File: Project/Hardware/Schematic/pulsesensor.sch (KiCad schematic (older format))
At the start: 2 parts, among them U4 Pulse_sensor

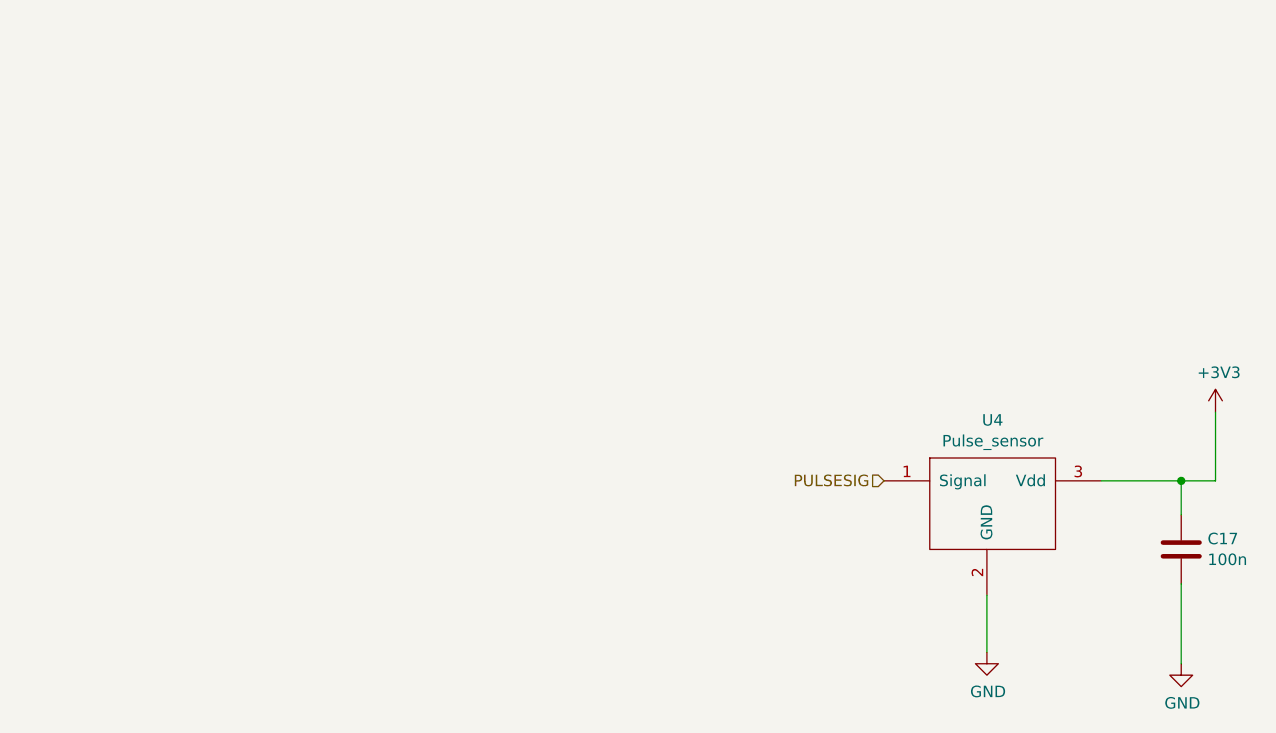
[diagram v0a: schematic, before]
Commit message: Intermediate...
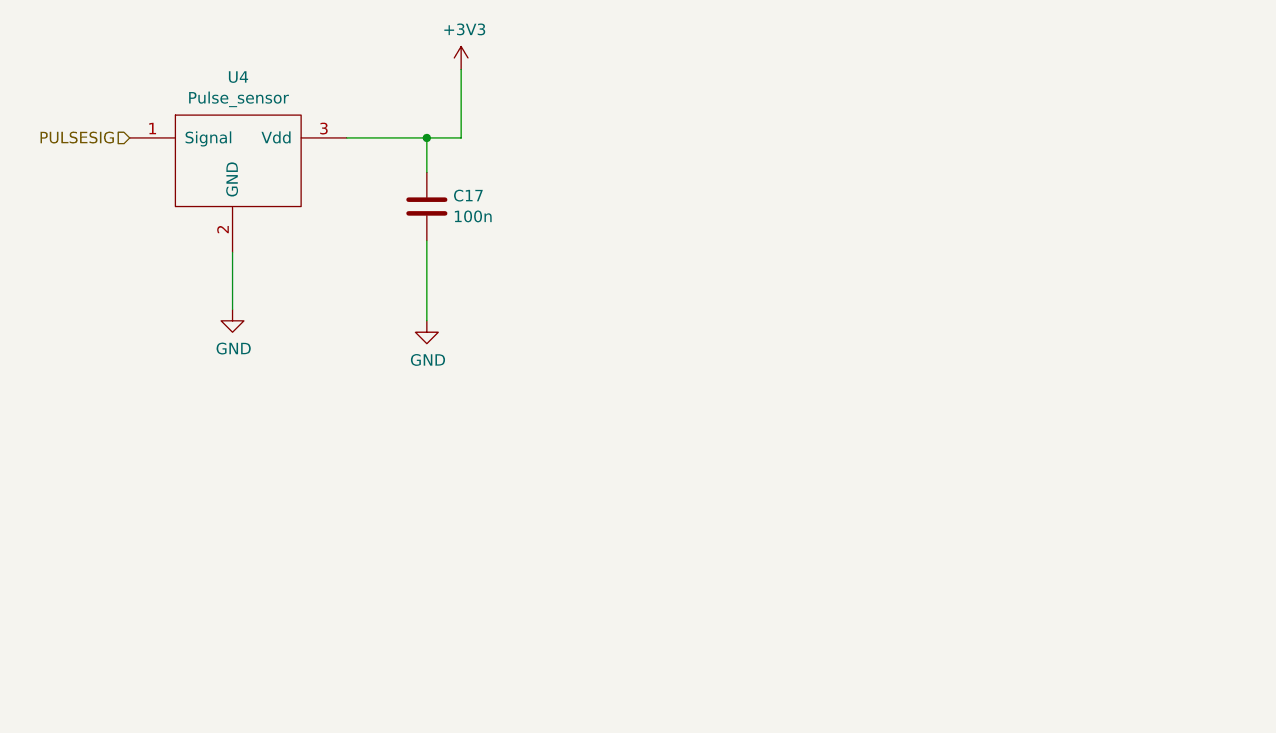
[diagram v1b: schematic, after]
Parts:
- C17: footprint (none) -> Capacitor_SMD:C_0805_2012Metric_Pad1.15x1.40mm_HandSolder
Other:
- moved on the sheet: C17, U4
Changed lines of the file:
@@
 EELAYER 26 0
 EELAYER END
-$Descr A4 11693 8268
+$Descr User 5512 5512
 encoding utf-8
 Sheet 3 7
 Title ""
-Date ""
-Rev ""
-Comp ""
+Date "2019-02-12"
+Rev "1"
+Comp "PASC"
 Comment1 ""
 Comment2 ""
@@
 L PASC:Pulse_sensor U4
 U 1 1 5C5DA663
-P 5700 3400
-F 0 "U4" H 5725 3765 50  0000 C CNN
-F 1 "Pulse_sensor" H 5725 3674 50  0000 C CNN
-F 2 "Pin_Headers:Pin_Header_Straight_1x03_Pitch2.54mm" H 5700 3400 50  0001 C CNN
-F 3 "" H 5700 3400 50  0001 C CNN
-	1    5700 3400
+P 2400 1900
+F 0 "U4" H 2425 2265 50  0000 C CNN
+F 1 "Pulse_sensor" H 2425 2174 50  0000 C CNN
+F 2 "Pin_Headers:Pin_Header_Straight_1x03_Pitch2.54mm" H 2400 1900 50  0001 C CNN
+F 3 "" H 2400 1900 50  0001 C CNN
+	1    2400 1900
 	1    0    0    -1
 $EndComp
@@
 L power:+3V3 #PWR0125
 U 1 1 5C5DA797
-P 6700 3000
-F 0 "#PWR0125" H 6700 2850 50  0001 C CNN
-F 1 "+3V3" H 6715 3173 50  0000 C CNN
-F 2 "" H 6700 3000 50  0001 C CNN
-F 3 "" H 6700 3000 50  0001 C CNN
-	1    6700 3000
+P 3400 1500
+F 0 "#PWR0125" H 3400 1350 50  0001 C CNN
+F 1 "+3V3" H 3415 1673 50  0000 C CNN
+F 2 "" H 3400 1500 50  0001 C CNN
+F 3 "" H 3400 1500 50  0001 C CNN
+	1    3400 1500
 	1    0    0    -1
 $EndComp
@@
 L Device:C C17
 U 1 1 5C5DA7DA
-P 6550 3600
-F 0 "C17" H 6665 3646 50  0000 L CNN
-F 1 "100n" H 6665 3555 50  0000 L CNN
-F 2 "" H 6588 3450 50  0001 C CNN
-F 3 "~" H 6550 3600 50  0001 C CNN
-	1    6550 3600
+P 3250 2100
+F 0 "C17" H 3365 2146 50  0000 L CNN
+F 1 "100n" H 3365 2055 50  0000 L CNN
+F 2 "Capacitor_SMD:C_0805_2012Metric_Pad1.15x1.40mm_HandSolder" H 3288 1950 50  0001 C CNN
+F 3 "~" H 3250 2100 50  0001 C CNN
+	1    3250 2100
 	1    0    0    -1
 $EndComp
 Wire Wire Line
-	6200 3300 6550 3300
+	2900 1800 3250 1800
 Wire Wire Line
-	6700 3300 6700 3000
+	3400 1800 3400 1500
 $Comp
 L power:GND #PWR0126
 U 1 1 5C5DA906
-P 5700 4050
-F 0 "#PWR0126" H 5700 3800 50  0001 C CNN
-F 1 "GND" H 5705 3877 50  0000 C CNN
-F 2 "" H 5700 4050 50  0001 C CNN
-F 3 "" H 5700 4050 50  0001 C CNN
-	1    5700 4050
+P 2400 2550
+F 0 "#PWR0126" H 2400 2300 50  0001 C CNN
+F 1 "GND" H 2405 2377 50  0000 C CNN
+F 2 "" H 2400 2550 50  0001 C CNN
+F 3 "" H 2400 2550 50  0001 C CNN
+	1    2400 2550
 	1    0    0    -1
 $EndComp
@@
 L power:GND #PWR0127
 U 1 1 5C5DA96D
-P 6550 4100
-F 0 "#PWR0127" H 6550 3850 50  0001 C CNN
-F 1 "GND" H 6555 3927 50  0000 C CNN
-F 2 "" H 6550 4100 50  0001 C CNN
-F 3 "" H 6550 4100 50  0001 C CNN
-	1    6550 4100
+P 3250 2600
+F 0 "#PWR0127" H 3250 2350 50  0001 C CNN
+F 1 "GND" H 3255 2427 50  0000 C CNN
+F 2 "" H 3250 2600 50  0001 C CNN
+F 3 "" H 3250 2600 50  0001 C CNN
+	1    3250 2600
 	1    0    0    -1
 $EndComp
 Wire Wire Line
-	6550 3750 6550 4100
+	3250 2250 3250 2600
 Wire Wire Line
-	6550 3450 6550 3300
-Connection ~ 6550 3300
+	3250 1950 3250 1800
+Connection ~ 3250 1800
 Wire Wire Line
-	6550 3300 6700 3300
+	3250 1800 3400 1800
 Wire Wire Line
-	5700 3800 5700 4050
-Text HLabel 5250 3300 0    50   Input ~ 0
+	2400 2300 2400 2550
+Text HLabel 1950 1800 0    50   Input ~ 0
 PULSESIG
 $EndSCHEMATC
